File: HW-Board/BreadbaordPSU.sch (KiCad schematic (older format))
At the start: 18 parts, among them J1 vin, J2 Outputs, Q1 Si4435, U1 MAX6241

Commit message: SYNC
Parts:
- D1: value D_Zener -> 10V
- Q1: symbol Peters:Si4435 -> BreadbaordPSU-rescue:Si4435-Peters
- R1: value R -> 100k
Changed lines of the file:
@@
 	4150 1550 4250 1550
 $Comp
-L Peters:Si4435 Q1
+L BreadbaordPSU-rescue:Si4435-Peters Q1
 U 1 1 5CF021A1
 P 2300 1350
@@
 P 2650 1400
 F 0 "D1" V 2604 1479 50  0000 L CNN
-F 1 "D_Zener" V 2695 1479 50  0000 L CNN
+F 1 "10V" V 2695 1479 50  0000 L CNN
 F 2 "" H 2650 1400 50  0001 C CNN
 F 3 "~" H 2650 1400 50  0001 C CNN
@@
 P 2300 1700
 F 0 "R1" H 2370 1746 50  0000 L CNN
-F 1 "R" H 2370 1655 50  0000 L CNN
+F 1 "100k" H 2370 1655 50  0000 L CNN
 F 2 "" V 2230 1700 50  0001 C CNN
 F 3 "~" H 2300 1700 50  0001 C CNN

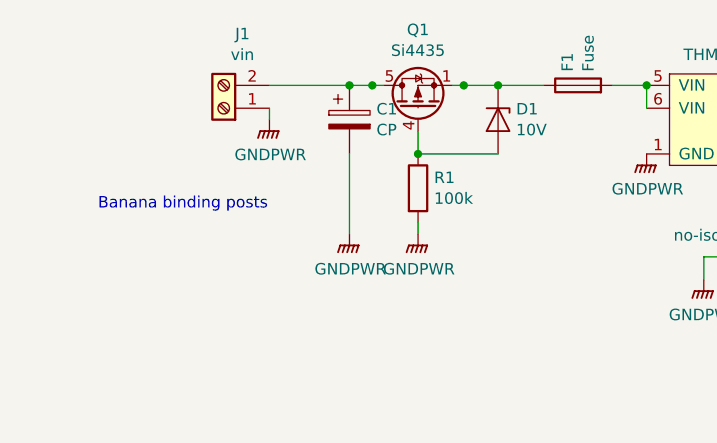
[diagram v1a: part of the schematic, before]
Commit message: sync
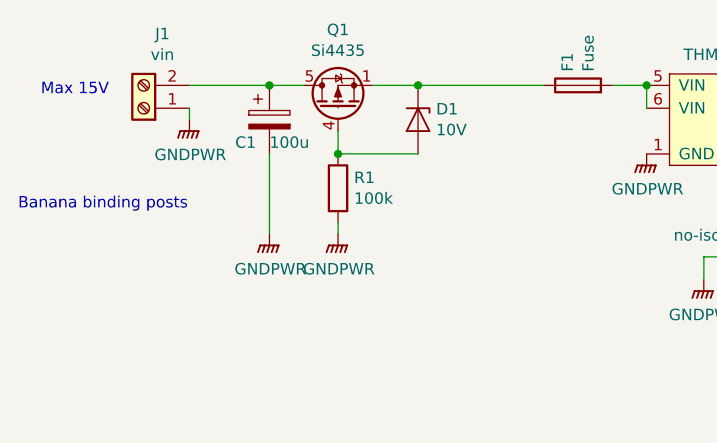
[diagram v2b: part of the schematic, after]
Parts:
- C1: value CP -> 100u
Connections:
- net at D1.1 (K), F1.1, Q1.1 (S): no longer Q1.2 (S), Q1.3 (S)
- net at C1.1, J1.2 (Pin_2), Q1.5 (D): no longer Q1.6 (D), Q1.7 (D), Q1.8 (D)
- new net: Q1.2 (S), Q1.3 (S)
- new net: Q1.6 (D), Q1.7 (D), Q1.8 (D)
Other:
- note added: "Max 15V"
- moved on the sheet: C1, D1, J1, Q1, R1
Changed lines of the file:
@@
 L Connector:Screw_Terminal_01x02 J1
 U 1 1 5CF83871
-P 1450 1350
-F 0 "J1" H 1368 1025 50  0000 C CNN
-F 1 "vin" H 1368 1116 50  0000 C CNN
-F 2 "" H 1450 1350 50  0001 C CNN
-F 3 "~" H 1450 1350 50  0001 C CNN
-	1    1450 1350
+P 1100 1350
+F 0 "J1" H 1018 1025 50  0000 C CNN
+F 1 "vin" H 1018 1116 50  0000 C CNN
+F 2 "" H 1100 1350 50  0001 C CNN
+F 3 "~" H 1100 1350 50  0001 C CNN
+	1    1100 1350
 	-1   0    0    1
 $EndComp
@@
 L power:GNDPWR #PWR0105
 U 1 1 5CF84A70
-P 1650 1400
-F 0 "#PWR0105" H 1650 1200 50  0001 C CNN
-F 1 "GNDPWR" H 1654 1246 50  0000 C CNN
-F 2 "" H 1650 1350 50  0001 C CNN
-F 3 "" H 1650 1350 50  0001 C CNN
-	1    1650 1400
-	1    0    0    -1
-$EndComp
-Wire Wire Line
-	1650 1350 1650 1400
+P 1300 1400
+F 0 "#PWR0105" H 1300 1200 50  0001 C CNN
+F 1 "GNDPWR" H 1304 1246 50  0000 C CNN
+F 2 "" H 1300 1350 50  0001 C CNN
+F 3 "" H 1300 1350 50  0001 C CNN
+	1    1300 1400
+	1    0    0    -1
+$EndComp
+Wire Wire Line
+	1300 1350 1300 1400
 $Comp
 L power:+12V #PWR0106
@@
 L BreadbaordPSU-rescue:Si4435-Peters Q1
 U 1 1 5CF021A1
-P 2300 1350
-F 0 "Q1" V 2643 1350 50  0000 C CNN
-F 1 "Si4435" V 2552 1350 50  0000 C CNN
-F 2 "Package_SO:SOIC-8_3.9x4.9mm_P1.27mm" H 2050 1650 50  0001 C CNN
-F 3 "https://www.vishay.com/docs/72123/72123.pdf" H 2150 1750 50  0001 C CNN
-	1    2300 1350
+P 1950 1350
+F 0 "Q1" V 2293 1350 50  0000 C CNN
+F 1 "Si4435" V 2202 1350 50  0000 C CNN
+F 2 "Package_SO:SOIC-8_3.9x4.9mm_P1.27mm" H 1700 1650 50  0001 C CNN
+F 3 "https://www.vishay.com/docs/72123/72123.pdf" H 1800 1750 50  0001 C CNN
+	1    1950 1350
 	0    -1   -1   0
 $EndComp
@@
 L Device:D_Zener D1
 U 1 1 5CF032D9
-P 2650 1400
-F 0 "D1" V 2604 1479 50  0000 L CNN
-F 1 "10V" V 2695 1479 50  0000 L CNN
-F 2 "" H 2650 1400 50  0001 C CNN
-F 3 "~" H 2650 1400 50  0001 C CNN
-	1    2650 1400
+P 2300 1400
+F 0 "D1" V 2254 1479 50  0000 L CNN
+F 1 "10V" V 2345 1479 50  0000 L CNN
+F 2 "" H 2300 1400 50  0001 C CNN
+F 3 "~" H 2300 1400 50  0001 C CNN
+	1    2300 1400
 	0    1    1    0
 $EndComp
@@
 L Device:R R1
 U 1 1 5CF126E3
-P 2300 1700
-F 0 "R1" H 2370 1746 50  0000 L CNN
-F 1 "100k" H 2370 1655 50  0000 L CNN
-F 2 "" V 2230 1700 50  0001 C CNN
-F 3 "~" H 2300 1700 50  0001 C CNN
-	1    2300 1700
-	1    0    0    -1
-$EndComp
-Wire Wire Line
-	2300 1450 2300 1550
-Wire Wire Line
-	2450 1250 2500 1250
-Connection ~ 2500 1250
-Wire Wire Line
-	2500 1250 2650 1250
-Wire Wire Line
-	2650 1550 2300 1550
-Connection ~ 2300 1550
+P 1950 1700
+F 0 "R1" H 2020 1746 50  0000 L CNN
+F 1 "100k" H 2020 1655 50  0000 L CNN
+F 2 "" V 1880 1700 50  0001 C CNN
+F 3 "~" H 1950 1700 50  0001 C CNN
+	1    1950 1700
+	1    0    0    -1
+$EndComp
+Wire Wire Line
+	1950 1450 1950 1550
+Wire Wire Line
+	2300 1550 1950 1550
+Connection ~ 1950 1550
 $Comp
 L power:GNDPWR #PWR0108
 U 1 1 5CF32200
-P 2300 1900
-F 0 "#PWR0108" H 2300 1700 50  0001 C CNN
-F 1 "GNDPWR" H 2304 1746 50  0000 C CNN
-F 2 "" H 2300 1850 50  0001 C CNN
-F 3 "" H 2300 1850 50  0001 C CNN
-	1    2300 1900
-	1    0    0    -1
-$EndComp
-Wire Wire Line
-	2300 1850 2300 1900
-Wire Wire Line
-	2150 1250 2100 1250
-Connection ~ 2100 1250
-Wire Wire Line
-	2100 1250 2000 1250
+P 1950 1900
+F 0 "#PWR0108" H 1950 1700 50  0001 C CNN
+F 1 "GNDPWR" H 1954 1746 50  0000 C CNN
+F 2 "" H 1950 1850 50  0001 C CNN
+F 3 "" H 1950 1850 50  0001 C CNN
+	1    1950 1900
+	1    0    0    -1
+$EndComp
+Wire Wire Line
+	1950 1850 1950 1900
 $Comp
 L Device:CP C1
 U 1 1 5CF42D89
-P 2000 1400
-F 0 "C1" H 2118 1446 50  0000 L CNN
-F 1 "CP" H 2118 1355 50  0000 L CNN
-F 2 "" H 2038 1250 50  0001 C CNN
-F 3 "~" H 2000 1400 50  0001 C CNN
-	1    2000 1400
+P 1650 1400
+F 0 "C1" H 1500 1300 50  0000 L CNN
+F 1 "100u" H 1650 1300 50  0000 L CNN
+F 2 "" H 1688 1250 50  0001 C CNN
+F 3 "~" H 1650 1400 50  0001 C CNN
+	1    1650 1400
 	1    0    0    -1
 $EndComp
@@
 L power:GNDPWR #PWR0109
 U 1 1 5CF437BA
-P 2000 1900
-F 0 "#PWR0109" H 2000 1700 50  0001 C CNN
-F 1 "GNDPWR" H 2004 1746 50  0000 C CNN
-F 2 "" H 2000 1850 50  0001 C CNN
-F 3 "" H 2000 1850 50  0001 C CNN
-	1    2000 1900
-	1    0    0    -1
-$EndComp
-Wire Wire Line
-	2000 1550 2000 1900
-Wire Wire Line
-	1650 1250 2000 1250
-Connection ~ 2000 1250
+P 1650 1900
+F 0 "#PWR0109" H 1650 1700 50  0001 C CNN
+F 1 "GNDPWR" H 1654 1746 50  0000 C CNN
+F 2 "" H 1650 1850 50  0001 C CNN
+F 3 "" H 1650 1850 50  0001 C CNN
+	1    1650 1900
+	1    0    0    -1
+$EndComp
+Wire Wire Line
+	1650 1550 1650 1900
+Wire Wire Line
+	1300 1250 1650 1250
+Connection ~ 1650 1250
 Wire Wire Line
 	3150 1250 3300 1250
-Wire Wire Line
-	2850 1250 2650 1250
-Connection ~ 2650 1250
+Connection ~ 2300 1250
 $Comp
 L Mechanical:MountingHole H1
@@
 	1    0    0    -1
 $EndComp
-Text Notes 900  1800 0    50   ~ 0
+Text Notes 550  1800 0    50   ~ 0
 Banana binding posts
 Text Notes 8500 5100 0    50   ~ 0
@@
 Text Notes 1400 6500 0    50   ~ 0
 Todo:\n\nMerge to fewer opamps\nex. OPA2189IDR
+Text Notes 650  1300 0    50   ~ 0
+Max 15V
+Wire Wire Line
+	1650 1250 1800 1250
+Wire Wire Line
+	2100 1250 2300 1250
+Wire Wire Line
+	2300 1250 2850 1250
 $EndSCHEMATC
